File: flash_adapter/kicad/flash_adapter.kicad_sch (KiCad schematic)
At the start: 14 parts, among them J1 Conn_01x10, J2 Conn_01x10, J3 DS1044-160G

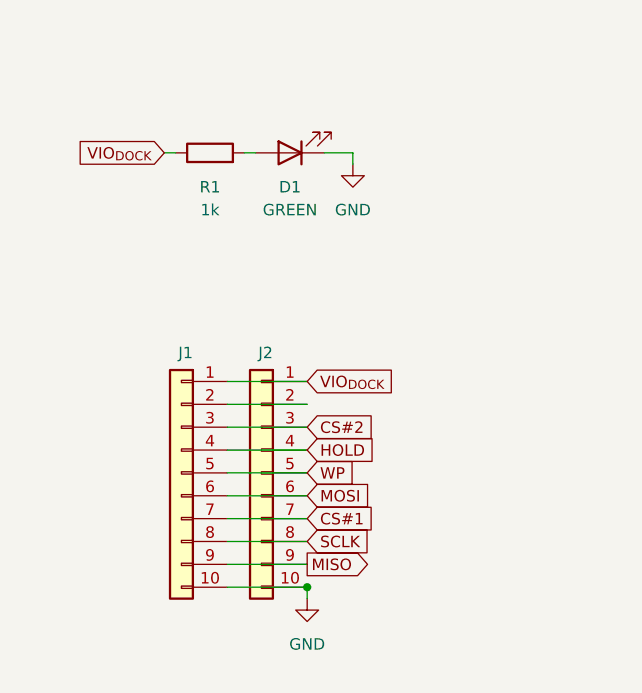
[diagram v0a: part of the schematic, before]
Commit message: Finished routing
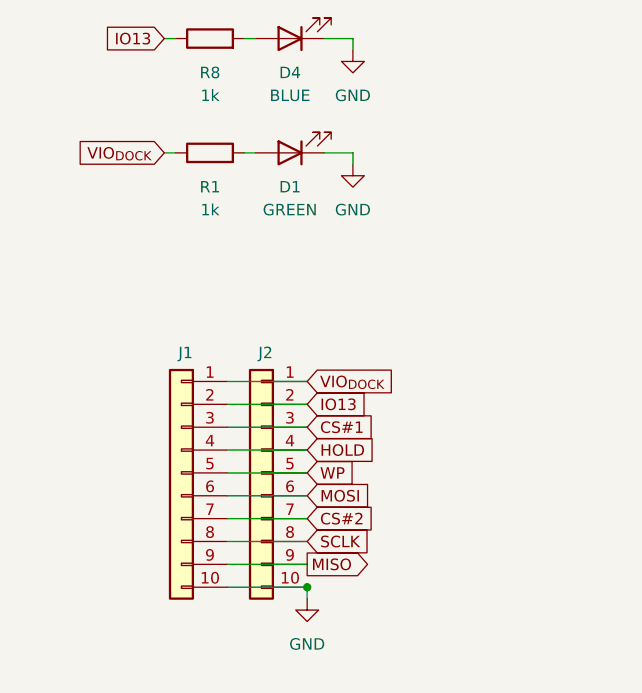
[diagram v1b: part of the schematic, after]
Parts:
- added D4: BLUE, LED_SMD:LED_0805_2012Metric, symbol Device:LED
- added R8: 1k, Resistor_SMD:R_0805_2012Metric, symbol Device:R
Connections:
- net CS#1: now also J1.3 (Pin_3), J2.3 (Pin_3); no longer J1.7 (Pin_7), J2.7 (Pin_7)
- net CS#2: now also J1.7 (Pin_7), J2.7 (Pin_7); no longer J1.3 (Pin_3), J2.3 (Pin_3)
- net GND: now also D4.1 (K)
- net IO13: now reaches J1.2 (Pin_2), J2.2 (Pin_2)
- net IO13: now also R8.1
- new net: D4.2 (A), R8.2
